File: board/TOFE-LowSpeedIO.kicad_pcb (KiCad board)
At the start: 2 copper layers, 1 part

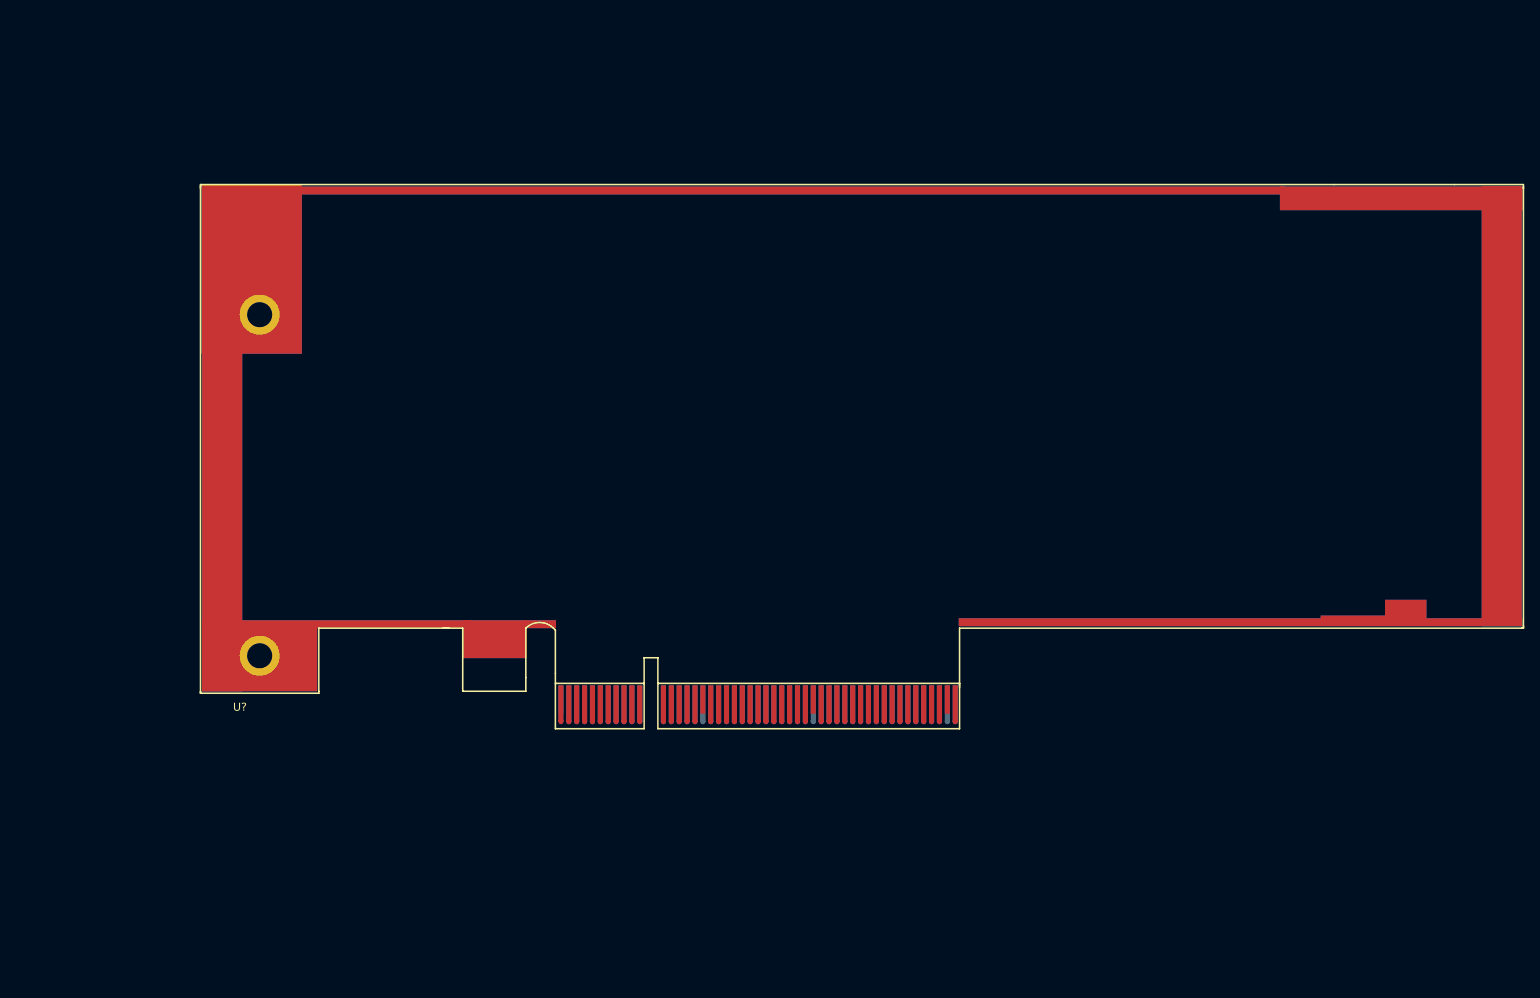
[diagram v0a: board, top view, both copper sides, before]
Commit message: Creating TOFE-LowSpeedIO!
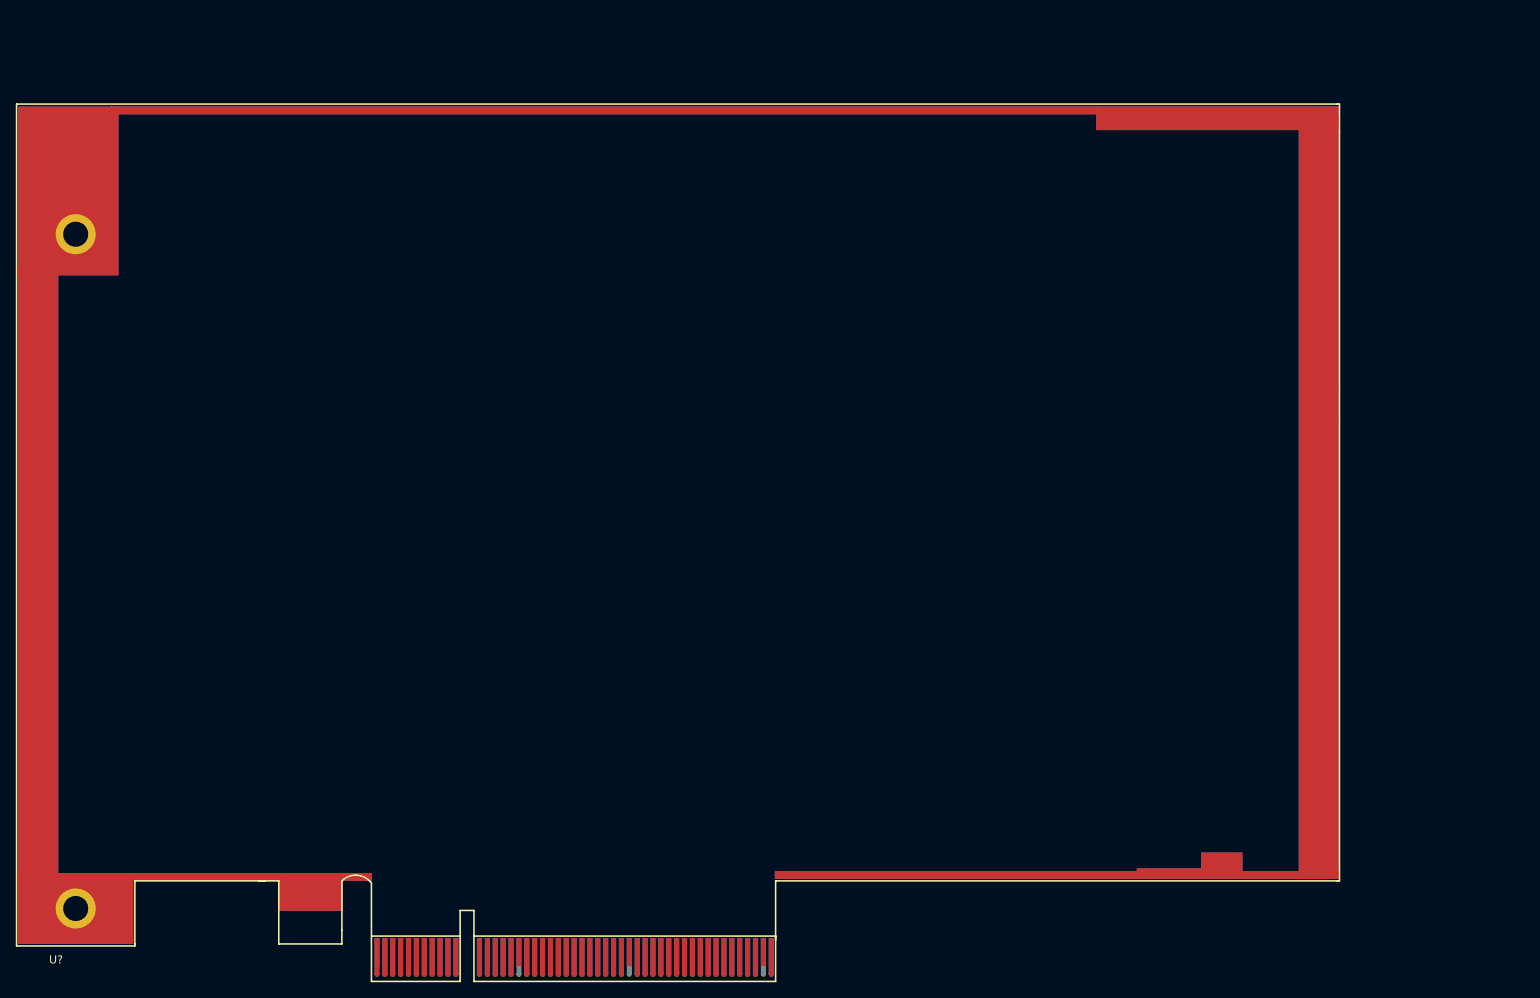
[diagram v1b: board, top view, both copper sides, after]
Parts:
- removed the U? at (148.4, 164.6)
- added U?: TOFE_LowSpeedIO_Expansion_Board_8x_FullHeight, TOFE_8X_FullHeight, F.Cu at (125.1, 196.7)

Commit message: Initial drop of TOFE LowSpeedIO Expansion Board.
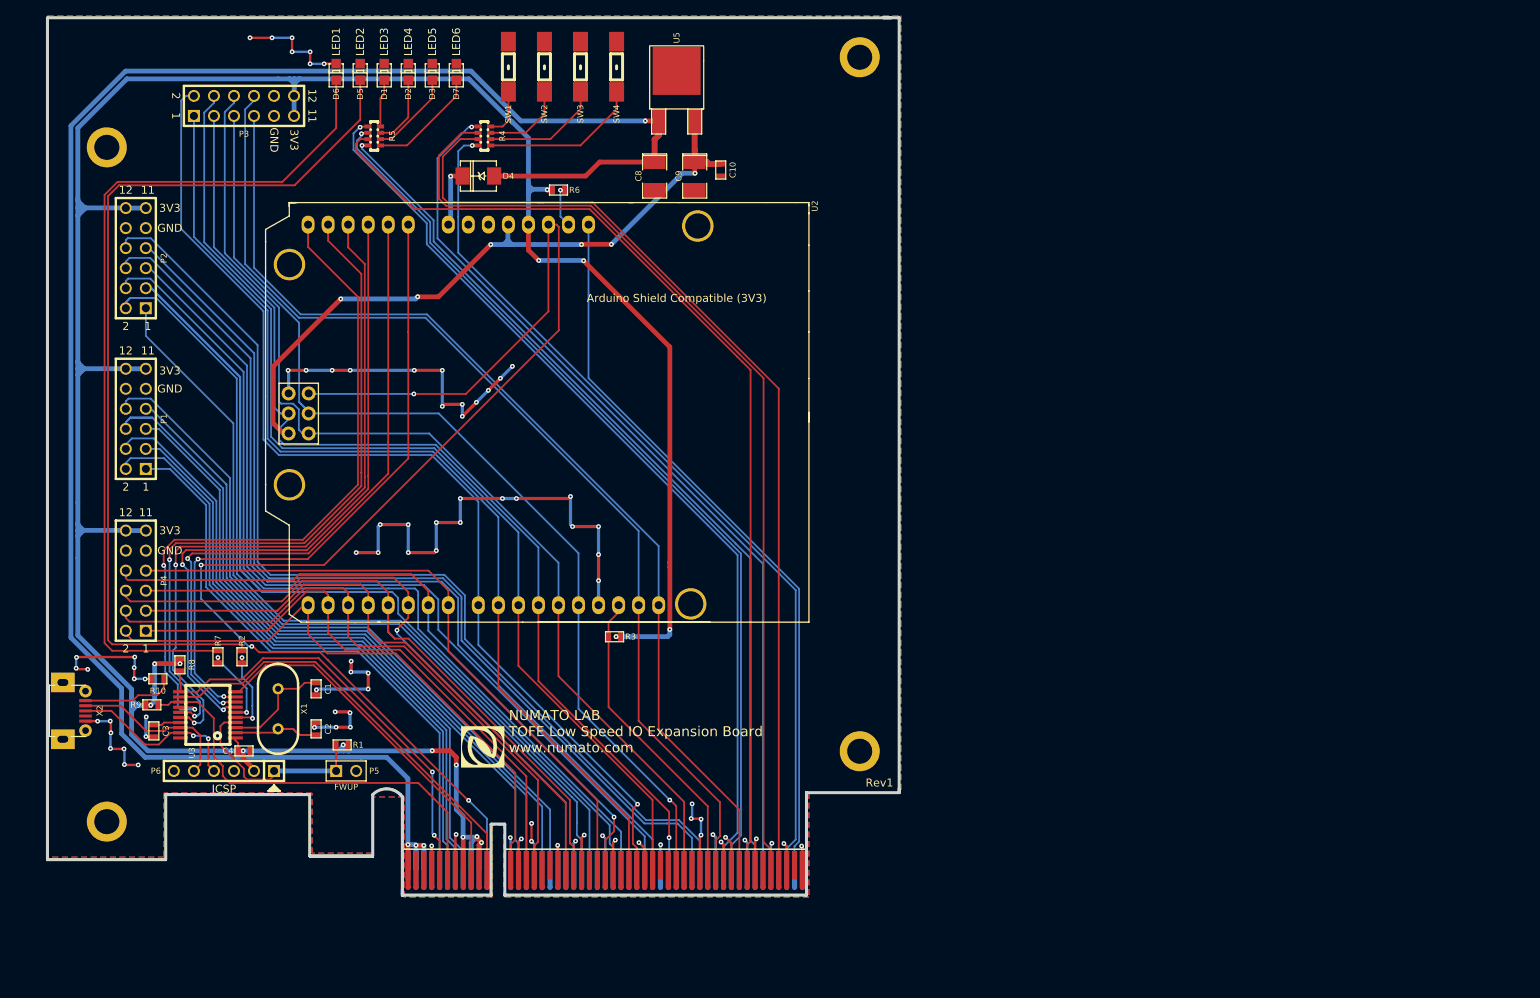
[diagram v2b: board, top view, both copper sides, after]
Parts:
- removed U?: TOFE_LowSpeedIO_Expansion_Board_8x_FullHeight, TOFE_8X_FullHeight
- added 1PIN: P***, MH-3.2MM, F.Cu at (232.0, 84.0)
- added 1PIN: P***, MH-3.2MM, F.Cu at (232.0, 172.0)
- added C1: 22pF, SM0603, F.Cu at (163.1, 164.1)
- added C10: 0.1uF, SM0603, F.Cu at (214.4, 98.3)
- added C2: 22pF, SM0603, F.Cu at (163.1, 169.2)
- added C3: 0.1uF, SM0603, F.Cu at (142.5, 169.4)
- added C4: 0.1uF, SM0603, F.Cu at (153.9, 172.0)
- added C8: 100uF, SM1210L, F.Cu at (206.0, 99.1)
- added C9: 100uF, SM1210L, F.Cu at (211.1, 99.1)
- added D1: LED, LED-0805-New, F.Cu at (171.7, 85.9)
- added D2: LED, LED-0805-New, F.Cu at (174.8, 85.9)
- added D3: LED, LED-0805-New, F.Cu at (177.8, 85.9)
- added D4: DIODE, DO214, F.Cu at (183.6, 99.1)
- added D5: LED, LED-0805-New, F.Cu at (168.7, 85.9)
- added D6: LED, LED-0805-New, F.Cu at (165.6, 85.9)
- added D7: LED, LED-0805-New, F.Cu at (180.8, 85.9)
- added G***: LOGO, LOGO_BOTTOM, F.Cu at (184.2, 171.4)
- added P1: CONN_6X2, pin_array_6x2, F.Cu at (140.2, 129.8)
- added P2: CONN_6X2, pin_array_6x2, F.Cu at (140.2, 109.5)
- added P3: CONN_6X2, pin_array_6x2, F.Cu at (153.9, 90.2)
- added P4: CONN_6X2, pin_array_6x2, F.Cu at (140.2, 150.4)
- added P5: CONN_2, PIN_ARRAY_2X1, F.Cu at (166.9, 174.5)
- added P6: CONN_6, PIN_ARRAY-6X1, F.Cu at (151.4, 174.5)
- added R1: 10K, SM0603, F.Cu at (166.4, 171.2)
- added R10: 100R, SM0603, F.Cu at (143.0, 162.8)
- added R2: 10K, SM0603, F.Cu at (153.7, 160.0)
- added R3: 10K, SM0603, F.Cu at (200.9, 157.5)
- added R4: 680R, RES_NET4, F.Cu at (184.4, 94.0)
- added R5: 10K, RES_NET4, F.Cu at (170.4, 94.0)
- added R6: 10K, SM0603, F.Cu at (193.8, 100.8)
- added R7: 10K, SM0603, F.Cu at (150.6, 160.0)
- added R8: 10K, SM0603, F.Cu at (145.8, 161.0)
- added R9: 10K, SM0603, F.Cu at (142.2, 166.1)
- added SW1: SW_PUSH, Switch_SMD, F.Cu at (187.5, 85.3)
- added SW2: SW_PUSH, Switch_SMD, F.Cu at (192.0, 85.3)
- added SW3: SW_PUSH, Switch_SMD, F.Cu at (196.6, 85.3)
- added SW4: SW_PUSH, Switch_SMD, F.Cu at (201.2, 85.3)
- added U1: TIMVIDEOS-PCIE-8X, NumatoOpsis_PCIe_8X_HL_NW, F.Cu at (129.0, 185.7)
- added U2: AURD_COMM_SHIELD_ZERO_NEW, ARDUINO-UNO-R3_1_NEW, F.Cu at (191.3, 129.0)
- added U3: PIC18F14K50, SSOP-20, F.Cu at (149.4, 167.4)
- added U5: 7805_NW, DPAK2, F.Cu at (208.8, 92.1)
- added X1: CRYSTAL, HC-49V, F.Cu at (158.2, 166.6)
- added X2: USBMICRO, MICRO_USB_B, F.Cu at (130.6, 166.9)
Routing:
- net /VCC3V3: track 0.00 -> 365.5 mm, vias 0 -> 15
- net /GND: track 0.00 -> 259.1 mm, vias 0 -> 87
- net /VCC12V: track 0.00 -> 244.6 mm, vias 0 -> 4
- net /RESET: track 0.00 -> 176.5 mm, vias 0 -> 4
- net /GPIO5_P: track 0.00 -> 169.8 mm
- net /D8: track 0.00 -> 135.1 mm, vias 0 -> 1
- net /D10: track 0.00 -> 133.4 mm
- net /D14: track 0.00 -> 133.1 mm
- net /D12: track 0.00 -> 133.0 mm
- net /D11: track 0.00 -> 132.4 mm, vias 0 -> 1
- net /D15: track 0.00 -> 130.4 mm
- net /D13: track 0.00 -> 130.2 mm, vias 0 -> 1
- net /D9: track 0.00 -> 129.7 mm
- net /GPIO7_N: track 0.00 -> 128.5 mm
- net /LED3: track 0.00 -> 127.7 mm
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- added copper zone on B.Cu, net /GND
- added copper zone on F.Cu, net /GND
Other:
- board outline added: 108 x 111.2 mm
- net class Default: clearance 0.254 -> 0.2032
- rule trace_clearance: 0.254 -> 0.2032
- rule trace_min: 0.254 -> 0.127
- rule via_min_drill: 0.508 -> 0.254
- rule via_min_size: 0.889 -> 0.4572
- board text added: "1"
- board text added: "11"
- board text added: "12"
- board text added: "2"
- board text added: "3V3"
- board text added: "Arduino Shield Compatible (3V3)"
- board text added: "FWUP"
- board text added: "GND"
- board text added: "ICSP"
- board text added: "LED1"
- board text added: "LED2"
- board text added: "LED3"
- board text added: "LED4"
- board text added: "LED5"
- board text added: "LED6"
- board text added: "NUMATO LAB TOFE Low Speed IO Expansion Board www.numato.com"
- board text added: "Rev1"

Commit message: Changes on 2015-11-03.
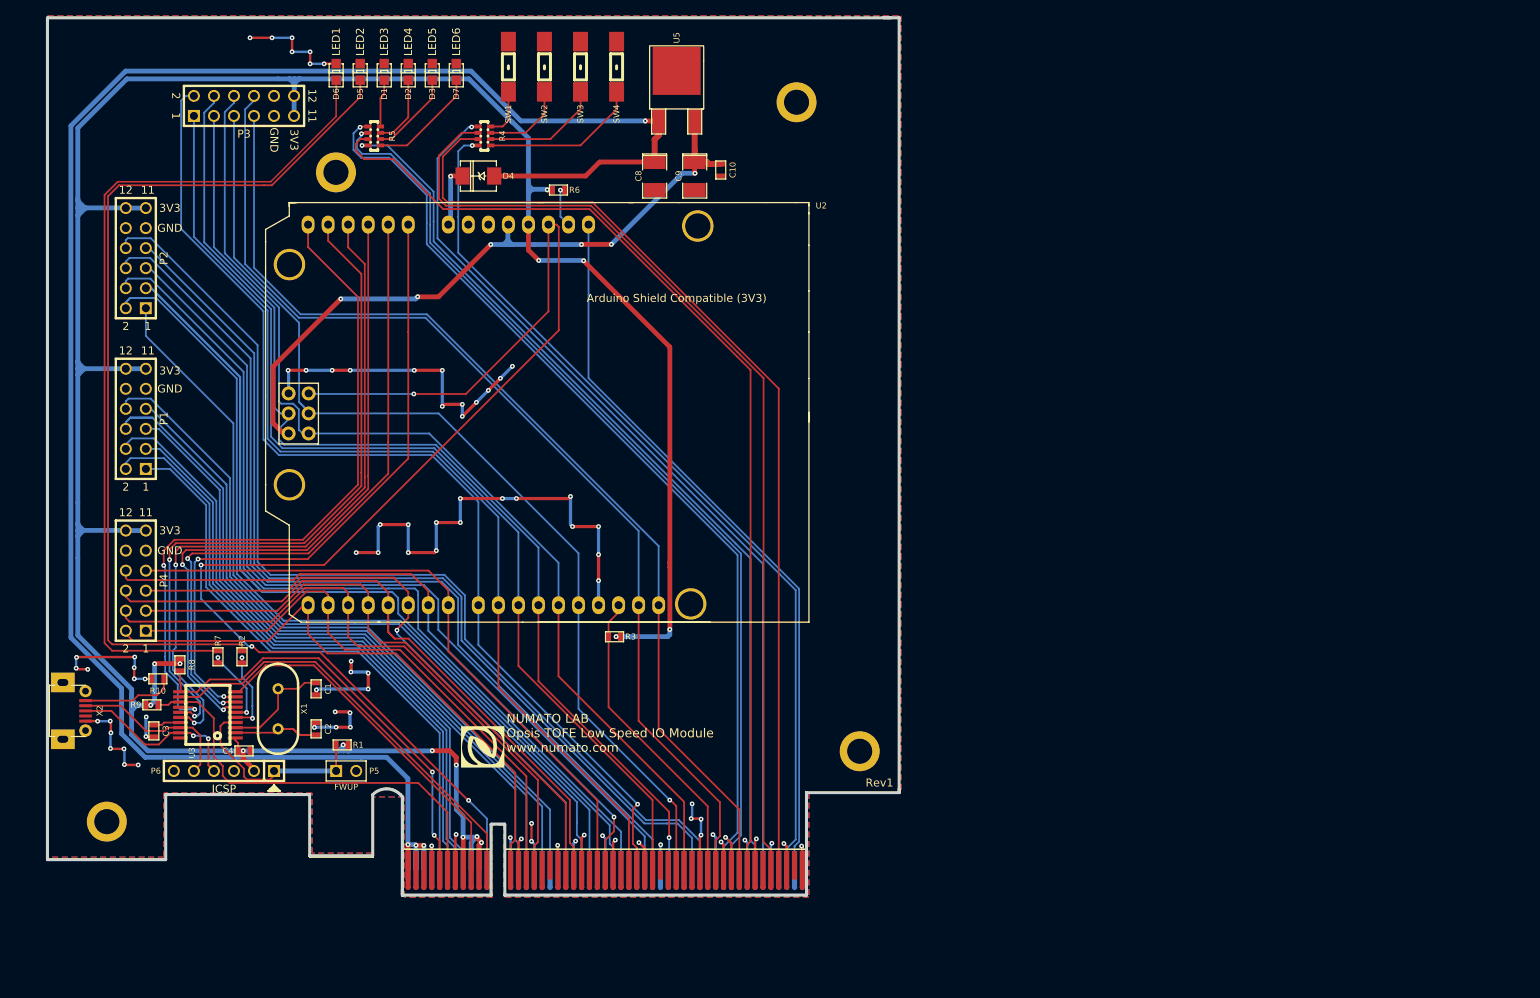
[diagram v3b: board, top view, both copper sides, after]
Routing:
- net /LED2: track 115.1 -> 117.2 mm
- net /LED1: track 116.5 -> 118.6 mm
- net /LED4: track 113.2 -> 115.1 mm
- net N-0000054: track 115.3 -> 113.6 mm
- net N-0000055: track 110.6 -> 109.7 mm
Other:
- net class Default: via_dia 0.889 -> 0.4572; via_drill 0.635 -> 0.254
- board text added: "NUMATO LAB Opsis TOFE Low Speed IO Module www.numato.com"
- board text removed: "NUMATO LAB TOFE Low Speed IO Expansion Board www.numato.com"
